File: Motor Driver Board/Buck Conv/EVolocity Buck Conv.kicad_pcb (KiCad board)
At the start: 4 copper layers, 120 x 90 mm, 53 parts, among them J1 Screw_Terminal_01x02, J2 XT30, J3 Screw_Terminal_01x02, J4 Conn_01x04, U1 NRF24L01_Breakout, U2 LM2576HVT-5, U4 L298N

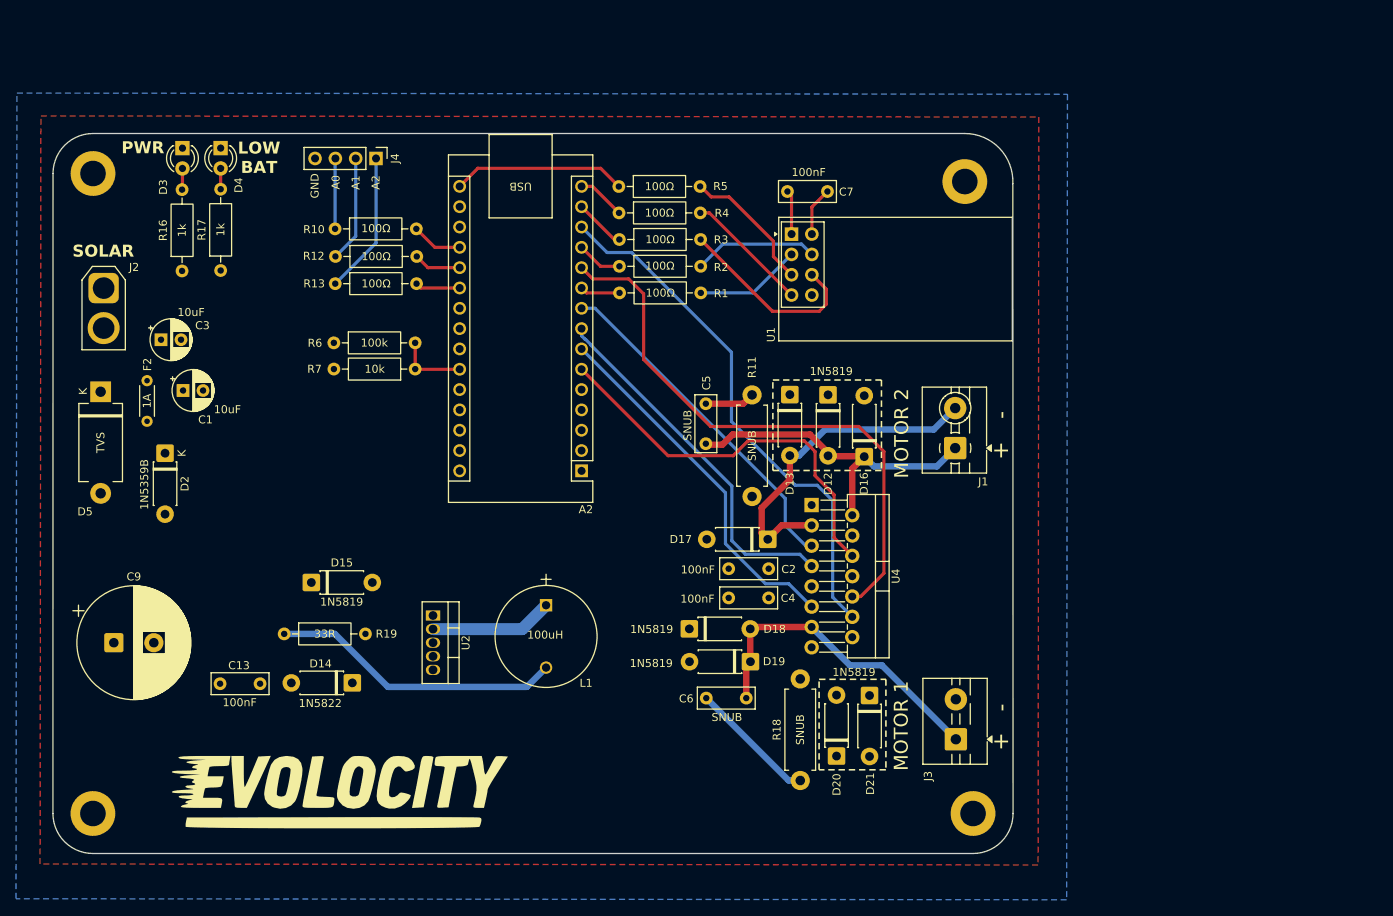
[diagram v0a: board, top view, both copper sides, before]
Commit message: updates maybe
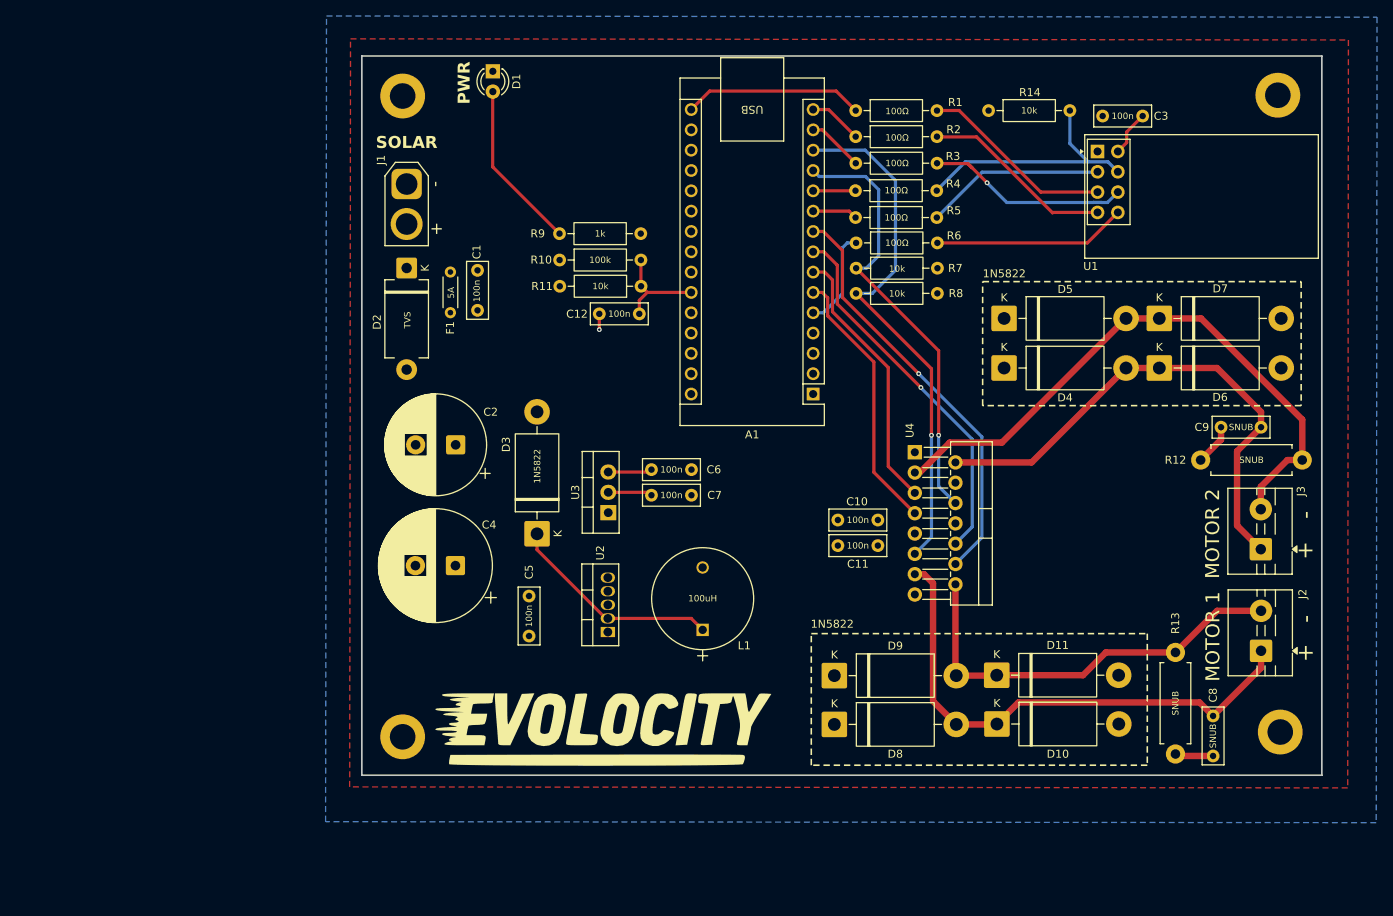
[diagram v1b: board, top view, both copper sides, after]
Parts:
- removed A2: Arduino_Nano_v3.x, Module:Arduino_Nano
- removed C13: 100nF, Capacitor_THT:C_Rect_L7.0mm_W2.5mm_P5.00mm
- removed D12, D13, D15, D16, D17, D18, D19, D20, D21: 1N5819, Diode_THT:D_DO-41_SOD81_P7.62mm_Horizontal
- removed D14: 1N5822, Diode_THT:D_DO-41_SOD81_P7.62mm_Horizontal
- removed F2: 1A, Resistor_THT:R_Axial_DIN0204_L3.6mm_D1.6mm_P5.08mm_Horizontal
- removed J4: Conn_01x04, Connector_PinHeader_2.54mm:PinHeader_1x04_P2.54mm_Vertical
- removed R16, R17: 1k, Resistor_THT:R_Axial_DIN0207_L6.3mm_D2.5mm_P10.16mm_Horizontal
- removed R18: R_snub, Resistor_THT:R_Axial_DIN0411_L9.9mm_D3.6mm_P12.70mm_Horizontal
- removed R19: 33R, Resistor_THT:R_Axial_DIN0207_L6.3mm_D2.5mm_P10.16mm_Horizontal
- added A1: Arduino Nano, Module:Arduino_Nano, F.Cu at (136.0, 98.3)
- added C10: 100nF, Capacitor_THT:C_Rect_L7.0mm_W2.5mm_P5.00mm, F.Cu at (144.1, 114.1)
- added C11: 100nF, Capacitor_THT:C_Rect_L7.0mm_W2.5mm_P5.00mm, F.Cu at (144.1, 117.3)
- added C12: 100nF, Capacitor_THT:C_Rect_L7.0mm_W2.5mm_P5.00mm, F.Cu at (114.3, 88.3)
- added C8: 100nF, Capacitor_THT:C_Rect_L7.0mm_W2.5mm_P5.00mm, F.Cu at (186.0, 138.6)
- added D1: Green, LED_THT:LED_D3.0mm_FlatTop, F.Cu at (96.0, 58.0)
- added D10: 1N5822, Diode_THT:D_DO-201AD_P15.24mm_Horizontal, F.Cu at (159.0, 139.6)
- added D11: 1N5822, Diode_THT:D_DO-201AD_P15.24mm_Horizontal, F.Cu at (159.0, 133.5)
- added D6: 1N5822, Diode_THT:D_DO-201AD_P15.24mm_Horizontal, F.Cu at (179.3, 95.1)
- added D7: 1N5822, Diode_THT:D_DO-201AD_P15.24mm_Horizontal, F.Cu at (179.3, 88.9)
- added D8: 1N5822, Diode_THT:D_DO-201AD_P15.24mm_Horizontal, F.Cu at (138.7, 139.6)
- added D9: 1N5822, Diode_THT:D_DO-201AD_P15.24mm_Horizontal, F.Cu at (138.7, 133.5)
- added F1: 5A, Resistor_THT:R_Axial_DIN0204_L3.6mm_D1.6mm_P5.08mm_Horizontal, F.Cu at (90.7, 83.1)
- added R14: 10k, Resistor_THT:R_Axial_DIN0207_L6.3mm_D2.5mm_P10.16mm_Horizontal, F.Cu at (157.9, 62.9)
- added R8: 10k, Resistor_THT:R_Axial_DIN0207_L6.3mm_D2.5mm_P10.16mm_Horizontal, F.Cu at (141.4, 85.7)
- added R9: 1k, Resistor_THT:R_Axial_DIN0207_L6.3mm_D2.5mm_P10.16mm_Horizontal, F.Cu at (114.5, 78.3)
- added U3: LD1117V33, Package_TO_SOT_THT:TO-220-3_Vertical, F.Cu at (110.4, 113.1)
- C1, C3: value 10uF -> 100nF; footprint Capacitor_THT:CP_Radial_D5.0mm_P2.50mm -> Capacitor_THT:C_Rect_L7.0mm_W2.5mm_P5.00mm
- C2: value 100nF -> 470uF; footprint Capacitor_THT:C_Rect_L7.0mm_W2.5mm_P5.00mm -> Capacitor_THT:CP_Radial_D12.5mm_P5.00mm
- C4: value 100nF -> 1000uF; footprint Capacitor_THT:C_Rect_L7.0mm_W2.5mm_P5.00mm -> Capacitor_THT:CP_Radial_D14.0mm_P5.00mm
- C5, C6: value C_Snub -> 100nF
- C7: value 100nF -> 10uF
- C9: value 100m -> 100nF; footprint Capacitor_THT:CP_Radial_D14.0mm_P5.00mm -> Capacitor_THT:C_Rect_L7.0mm_W2.5mm_P5.00mm
- D2: value 1N5359B -> 1.5KE39CA (TVS); footprint Diode_THT:D_DO-41_SOD81_P7.62mm_Horizontal -> Diode_THT:D_DO-201_P12.70mm_Horizontal
- D3: value Green -> 1N5822; footprint LED_THT:LED_D3.0mm_FlatTop -> Diode_THT:D_DO-201AD_P15.24mm_Horizontal
- D4: value Red -> 1N5822; footprint LED_THT:LED_D3.0mm_FlatTop -> Diode_THT:D_DO-201AD_P15.24mm_Horizontal
- D5: value 1.5KE39CA (TVS) -> 1N5822; footprint Diode_THT:D_DO-201_P12.70mm_Horizontal -> Diode_THT:D_DO-201AD_P15.24mm_Horizontal
- J1: value Screw_Terminal_01x02 -> XT30; footprint TerminalBlock:TerminalBlock_MaiXu_MX126-5.0-02P_1x02_P5.00mm -> Connector_AMASS:AMASS_XT30U-F_1x02_P5.0mm_Vertical
- J2: value XT30 -> Screw_Terminal_01x02; footprint Connector_AMASS:AMASS_XT30U-F_1x02_P5.0mm_Vertical -> TerminalBlock:TerminalBlock_MaiXu_MX126-5.0-02P_1x02_P5.00mm
- R1, R2, R3, R4, R5: value 100 -> 100R
- R10: value 100 -> 100k
- R11: value R_snub -> 10k; footprint Resistor_THT:R_Axial_DIN0411_L9.9mm_D3.6mm_P12.70mm_Horizontal -> Resistor_THT:R_Axial_DIN0207_L6.3mm_D2.5mm_P10.16mm_Horizontal
- R12, R13: value 100 -> 1k; footprint Resistor_THT:R_Axial_DIN0207_L6.3mm_D2.5mm_P10.16mm_Horizontal -> Resistor_THT:R_Axial_DIN0411_L9.9mm_D3.6mm_P12.70mm_Horizontal
- R6: value 100k -> 100R
- moved J2 151.6 mm to (192.0, 130.4), turned to 90 degrees
- moved H1 148.4 mm to (194.1, 61.0)
- moved C9 145.9 mm to (192.0, 102.5), turned to 180 degrees
- moved C3 125.8 mm to (177.2, 63.6), turned to 180 degrees
- moved R13 120.4 mm to (181.3, 143.3), turned to 90 degrees
- moved D5 113.3 mm to (159.9, 88.9), turned to 0 degrees
- moved R12 111.1 mm to (184.4, 106.6)
- moved D4 101.7 mm to (159.9, 95.1), turned to 0 degrees
- moved H4 98.8 mm to (84.7, 141.2)
- moved H2 97.7 mm to (84.7, 61.1)
- moved J1 76.1 mm to (85.2, 72.1), turned to -90 degrees
- moved R6 66.5 mm to (141.4, 79.4)
- moved D3 65.5 mm to (101.5, 115.8), turned to 90 degrees
- moved R7 56.5 mm to (141.4, 82.6), turned to 0 degrees
- moved J3 44.9 mm to (192.0, 117.7)
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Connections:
- C1 pad 1: +5V -> PowerInput+
- C2 pad 1: +5V -> PowerInput+
- C3 pad 1: +5V -> +3V3
- C5 pad 1: Net-(D12-A) -> +5V
- C5 pad 2: Net-(C5-Pad2) -> GND
- C6 pad 1: Net-(D18-A) -> +5V
- C6 pad 2: Net-(C6-Pad2) -> GND
- C9 pad 1: GND -> Net-(D4-A)
- C9 pad 2: +5V -> Net-(C9-Pad2)
- D2 pad 1: +5V -> PowerInput+
- D3 pad 1: GND -> Net-(D3-K)
- D3 pad 2: Net-(D3-A) -> GND
- D4 pad 1: GND -> PowerInput+
- D5 pad 1: Net-(D5-A1) -> PowerInput+
- D5 pad 2: GND -> Net-(D5-A)
- J1 pad 1: Net-(D12-A) -> GND
- J1 pad 2: Net-(D13-A) -> Net-(J1-Pin_2)
- J2 pad 1: GND -> Net-(D10-K)
- J2 pad 2: Net-(D5-A1) -> Net-(D11-K)
- J3 pad 1: Net-(D18-A) -> Net-(D4-A)
- J3 pad 2: Net-(D20-A) -> Net-(D5-A)
- L1 pad 1: Net-(D14-K) -> Net-(D3-K)
- L1 pad 2: Net-(L1-Pad2) -> +5V
- R1 pad 2: /Radio_CE -> /Radio_SCK
- R10 pad 1: /A0 -> PowerInput+
- R10 pad 2: Net-(A2-A0) -> /V_Panel_Analog
- R11 pad 1: Net-(C5-Pad2) -> /V_Panel_Analog
- R11 pad 2: Net-(D13-A) -> GND
- R12 pad 1: /A1 -> Net-(C9-Pad2)
- R12 pad 2: Net-(A2-A1) -> Net-(D5-A)
- R13 pad 1: /A2 -> Net-(C8-Pad2)
- R13 pad 2: Net-(A2-A2) -> Net-(D11-K)
- R2 pad 2: /Radio_CS -> /Radio_MISO
- R4 pad 2: /Radio_MISO -> /Radio_CS
- R5 pad 2: /Radio_SCK -> /Radio_CE
- R6 pad 1: +5V -> Net-(A1-D2)
- R6 pad 2: /V_Panel_Analog -> /Radio_IRQ
- R7 pad 1: /V_Panel_Analog -> /EnA
- U1 pad 8: unconnected-(U1-IRQ-Pad8) -> /Radio_IRQ
- U2 pad 1: +5V -> PowerInput+
- U2 pad 2: Net-(D14-K) -> Net-(D3-K)
- U2 pad 4: Net-(D14-K) -> +5V
- U2 pad 5: +5V -> GND
- U4 pad 13: Net-(D18-A) -> Net-(D10-K)
- U4 pad 14: Net-(D20-A) -> Net-(D11-K)
- U4 pad 2: Net-(D12-A) -> Net-(D4-A)
- U4 pad 3: Net-(D13-A) -> Net-(D5-A)
- U4 pad 4: +5V -> PowerInput+
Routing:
- net PowerInput+: track 0.00 -> 177.6 mm
- net +3V3: track 6.13 -> 109.2 mm
- net +5V: track 105.1 -> 13.7 mm
- net Net-(D5-A): track 0.00 -> 76.1 mm
- net Net-(D10-K): track 0.00 -> 66.2 mm
- net Net-(D4-A): track 2.60 -> 65.0 mm
- net Net-(D11-K): track 0.00 -> 52.9 mm
- net Net-(D12-A): track 42.3 -> 0.00 mm
- net Net-(D13-A): track 41.6 -> 0.00 mm
- net Net-(D18-A): track 40.5 -> 0.00 mm
- net Net-(L1-Pad2): track 36.5 -> 0.00 mm
- net Net-(D14-K): track 32.9 -> 0.00 mm
- net Net-(D20-A): track 28.0 -> 0.00 mm
- net Net-(D3-K): track 0.00 -> 26.8 mm
- net /IN3: track 72.5 -> 46.4 mm, vias 0 -> 1
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- removed copper zone on In2.Cu, net +3V3
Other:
- board size 120 x 90 mm -> 120 x 89.9 mm
- board text added: "100n"
- board text added: "5A"
- board text removed: "100nF"
- board text removed: "10uF"
- board text removed: "1A"
- board text removed: "1N5359B"
- board text removed: "1N5819"
- board text removed: "33R"
- board text removed: "A0"
- board text removed: "A1"
- board text removed: "A2"
- board text removed: "GND"
- board text removed: "LOW BAT"
